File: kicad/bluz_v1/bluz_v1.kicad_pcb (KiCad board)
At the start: 2 copper layers, 24.9 x 14.9 mm, 59 parts, among them J1 USB_B_Micro, J11 Conn, J12 BTAnt, J2 Conn, J3 Conn, J4 Conn, J5 Conn, J6 Conn, J7 Conn, J8 Conn, M1 VibroMotor, Q1 RUM002N05, Q2 RUM002N05, SW1 SW_DPDT_x2, U1 MCP73831, U2 MCP1700, U3 TLV3201AIDCK, Y1 NX2016SA-32MHz

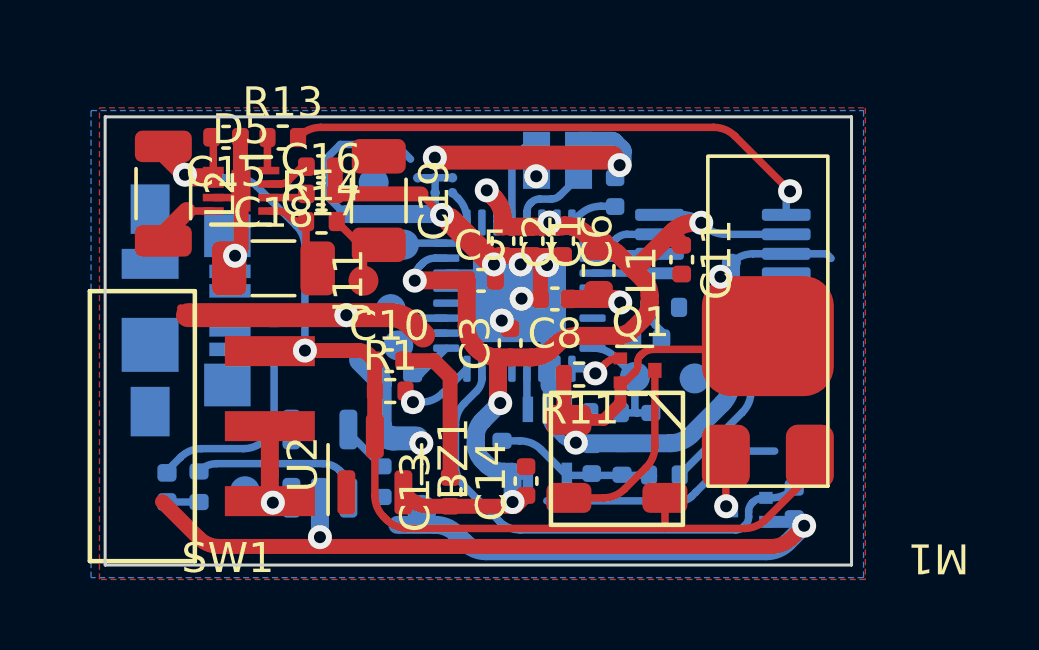
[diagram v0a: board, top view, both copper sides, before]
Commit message: удалено:       kicad/bluz_v1/bluz_v1-backups/bluz_v1-2024-04-19_190122.zip 	удалено:       kicad/bluz_v1/bluz_v1-backups/bluz_v1-2024-04-22_153028.zip 	удалено:       kicad/bluz_v1/bluz_v1-backups/bluz_v1-2024-04-26_142701.zip 	удалено:       kicad/bluz_v1/bluz_v1-backups/bluz_v1-2024-05-03_144119.zip 	удалено:       kicad/bluz_v1/bluz_v1-backups/bluz_v1-2024-05-03_145331.zip 	изменено:      kicad/bluz_v1/bluz_v1.kicad_pcb 	изменено:      kicad/bluz_v1/bluz_v1.kicad_sch 	изменено:      kicad/bluz_v1/fp-info-cache
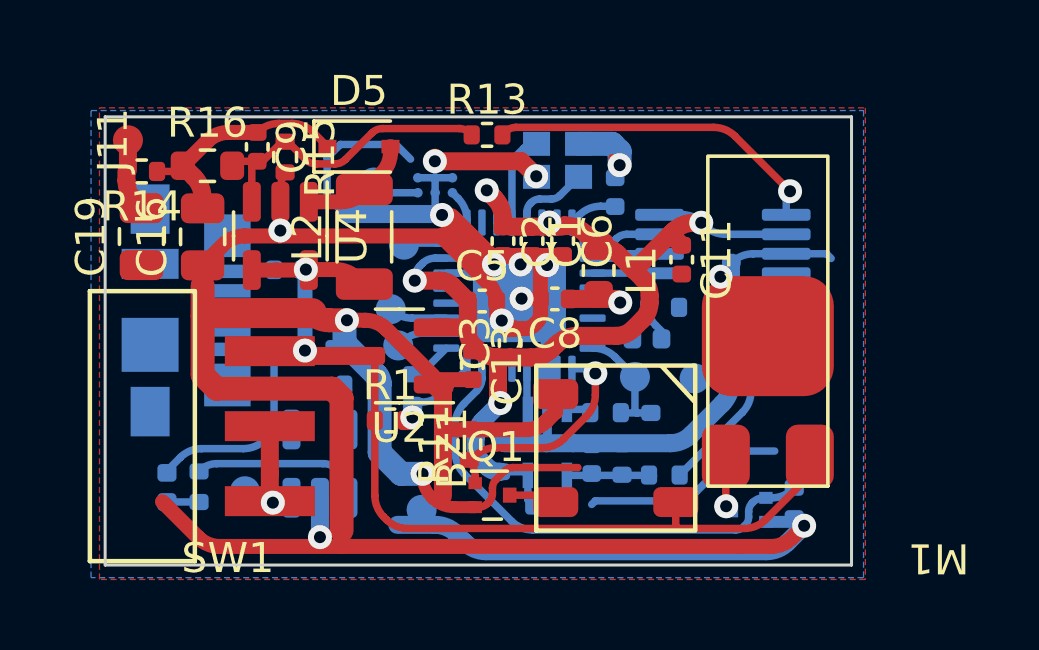
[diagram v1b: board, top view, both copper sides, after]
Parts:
- removed C17: .47, Capacitor_SMD:C_0402_1005Metric
- removed C18: 10u, Capacitor_SMD:C_1206_3216Metric
- added C9: 1.5p, Capacitor_SMD:C_0402_1005Metric, F.Cu at (66.8, 38.1)
- added R15: 4.3M, Resistor_SMD:R_0402_1005Metric, F.Cu at (67.7, 38.5)
- added R16: 100M, Resistor_SMD:R_0603_1608Metric, F.Cu at (65.1, 38.7)
- added U4: AP3015KTR, Package_TO_SOT_SMD:SOT-23-5, F.Cu at (67.5, 41.1)
- BZ1: footprint lib:Buzzer5x5 -> MyLibrary:Buzzer55x55
- C10, C14, C15: moved to B.Cu
- C16: value .47 -> 10u; footprint Capacitor_SMD:C_0402_1005Metric -> Capacitor_SMD:C_0805_2012Metric
- C19: footprint Capacitor_SMD:C_1206_3216Metric -> Capacitor_SMD:C_0805_2012Metric
- D5: value LT8410 -> BAT46JFILM; footprint Package_DFN_QFN:DFN-8-1EP_2x2mm_P0.45mm_EP0.64x1.38mm -> Diode_SMD:D_SOD-323
- L2: value 560uH -> 220uH
- R13: value R -> 100M
- U2: footprint Package_TO_SOT_SMD:SOT-23 -> Package_TO_SOT_SMD:SOT-23-3
- moved J11 9.14 mm to (62.5, 37.9)
- moved C19 8.00 mm to (62.9, 41.1), turned to 90 degrees
- moved L2 6.85 mm to (70.3, 41.1), turned to 90 degrees
- moved R13 6.81 mm to (74.4, 37.7)
- moved Q1 6.38 mm to (74.6, 49.7)
- moved R14 6.22 mm to (62.9, 38.9), turned to 180 degrees
- moved C15 4.88 mm to (67.8, 42.2), turned to 0 degrees
- moved R11 4.34 mm to (73.8, 48.0), turned to 90 degrees
- moved C13 4.28 mm to (73.9, 45.4), turned to -90 degrees
- moved D5 4.20 mm to (70.2, 38.1)
- moved C16 4.19 mm to (65.0, 41.1), turned to 90 degrees
- moved U2 3.70 mm to (71.5, 45.1), turned to 180 degrees
- moved R3 3.31 mm to (70.2, 46.0), turned to 0 degrees
- moved C10 2.36 mm to (68.8, 44.9)
- moved R9 2.25 mm to (76.5, 50.0), turned to 0 degrees
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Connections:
- C16 pad 1: Net-(C16-Pad1) -> GND
- C16 pad 2: GND -> Net-(C16-Pad2)
- D5 pad 1: +BATT -> Net-(C16-Pad2)
- D5 pad 2: +BATT -> Net-(D5-Pad2)
- L2 pad 2: Net-(D5-Pad4) -> Net-(D5-Pad2)
- R13 pad 1: Net-(D5-Pad8) -> Net-(C9-Pad2)
- R14 pad 1: Net-(C18-Pad2) -> Net-(C16-Pad2)
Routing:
- net GND: track 131.2 -> 153.9 mm, vias 16 -> 15
- net Net-(C9-Pad2): track 0.00 -> 10.5 mm
- net Net-(C16-Pad2): track 0.00 -> 8.16 mm
- net HVAdj: track 18.2 -> 11.3 mm
- net Sound: track 1.90 -> 7.63 mm
- net +BATT: track 36.3 -> 31.1 mm
- net Net-(BZ1-Pad1): track 6.25 -> 1.63 mm
- net Net-(D5-Pad2): track 0.00 -> 3.74 mm
- net +2V8: track 41.2 -> 37.7 mm, vias 6 -> 5
- net Net-(C18-Pad2): track 3.06 -> 0.00 mm
- net Net-(D5-Pad4): track 2.20 -> 0.00 mm
- net Net-(C12-Pad1): track 5.36 -> 3.80 mm
- net Net-(C17-Pad2): track 1.48 -> 0.00 mm
- net Net-(C16-Pad1): track 1.30 -> 0.00 mm
- net Net-(D5-Pad8): track 1.12 -> 0.00 mm
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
